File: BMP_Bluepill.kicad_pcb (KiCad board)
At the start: 2 copper layers, 42.3 x 20 mm, 30 parts, among them J1 Conn_01x06, J2 USB_C_Receptacle_USB2.0_16P, J3 Conn_01x04, U1 STM32F103C8T6, U2 AMS1117-3.3, Y1 8 MHz

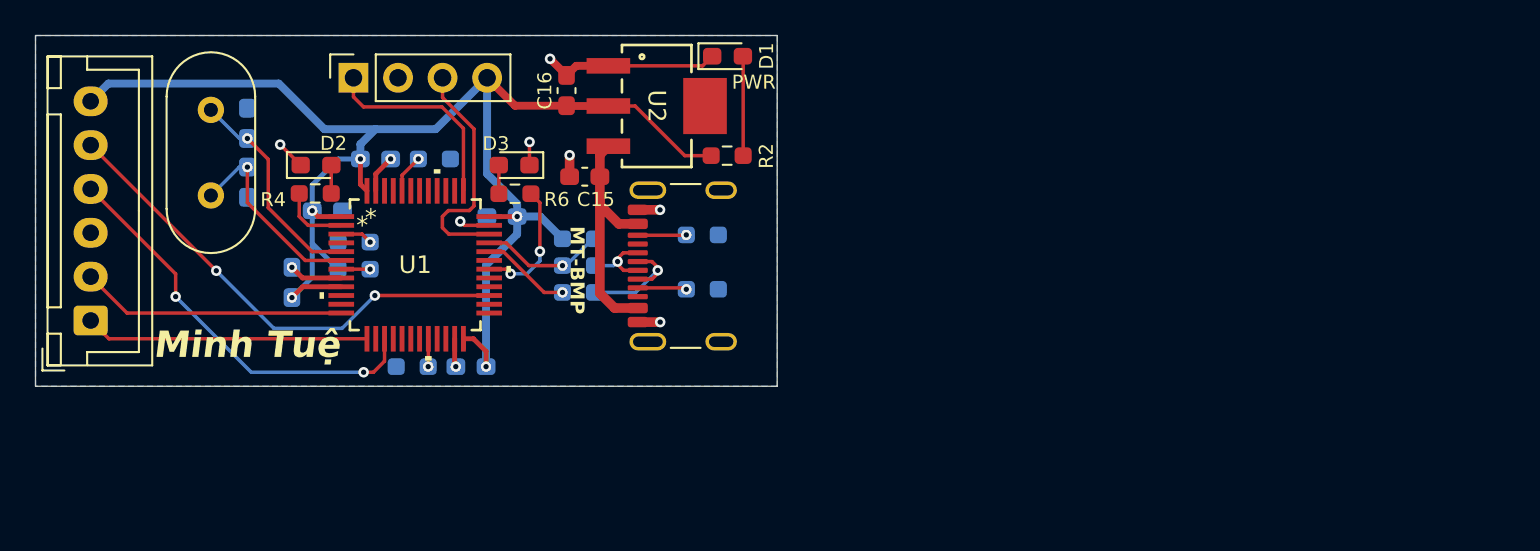
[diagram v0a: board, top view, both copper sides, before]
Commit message: fix layout
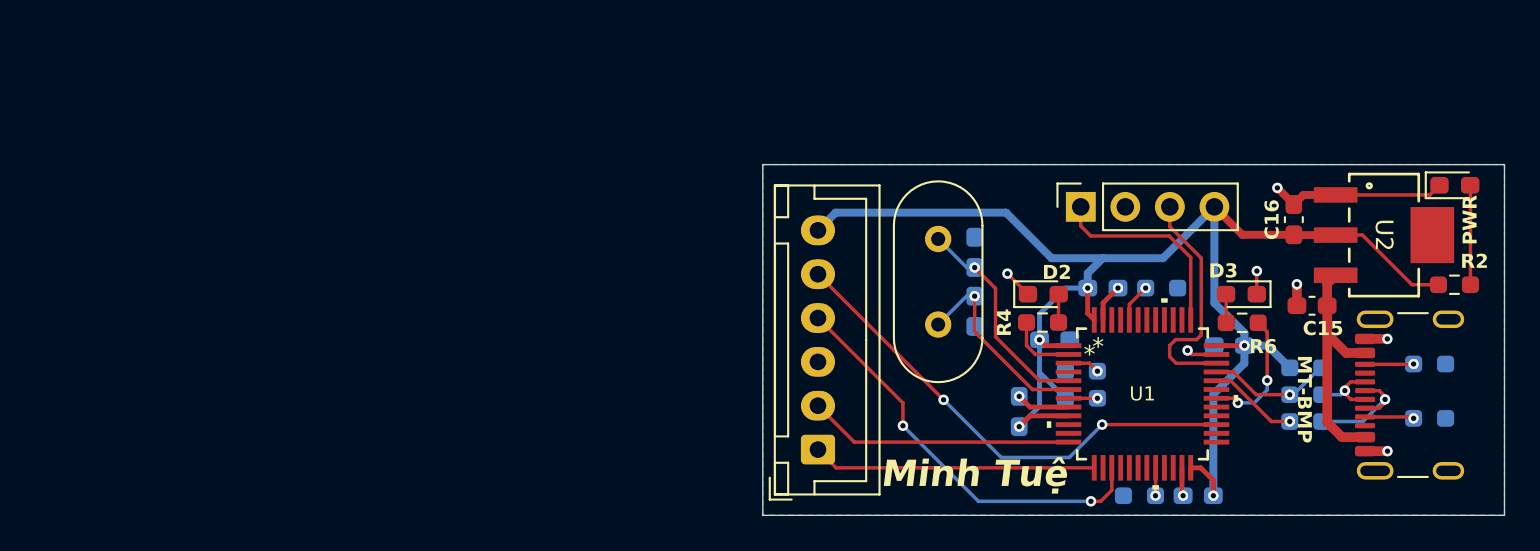
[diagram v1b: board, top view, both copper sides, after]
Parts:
- moved D1 42.1 mm to (139.5, 101.2)
- moved D2 42.1 mm to (116.0, 107.4)
- moved D3 42.1 mm to (127.3, 107.4)
- moved J2 42.1 mm to (138.0, 113.1)
- moved R12 42.1 mm to (131.0, 111.6)
- moved R16 42.1 mm to (131.0, 113.1)
- moved R17 42.1 mm to (131.0, 114.7)
- moved R18 42.1 mm to (138.0, 114.5)
- moved R19 42.1 mm to (138.0, 111.4)
- moved R7 42.1 mm to (121.5, 118.9)
- moved R8 42.1 mm to (122.7, 107.0)
- moved C1 42.1 mm to (126.6, 110.3)
- moved C13 42.1 mm to (112.1, 105.0)
- moved C14 42.1 mm to (112.1, 108.4)
- moved C15 42.1 mm to (131.3, 108.0)
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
